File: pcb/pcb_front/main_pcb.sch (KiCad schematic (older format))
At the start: 31 parts, among them J1 AVR-ISP-6, J2 USB_C_Receptacle, Q1 Q_NMOS_DGS, SW1 RESET, SW2 BOOT, SW3 BL_STEP, U1 ATmega32-16PU, Y1 Crystal

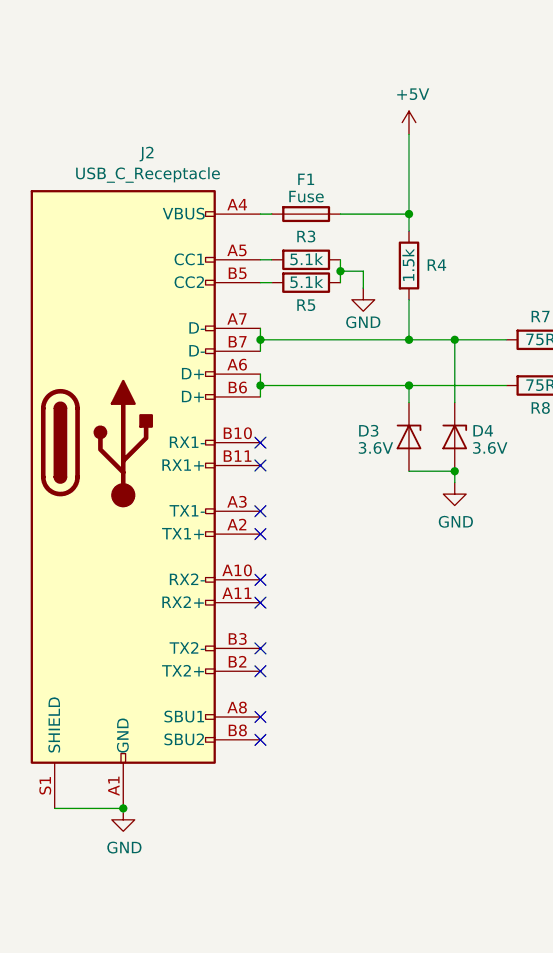
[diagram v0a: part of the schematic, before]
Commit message: Finish footprint assignments
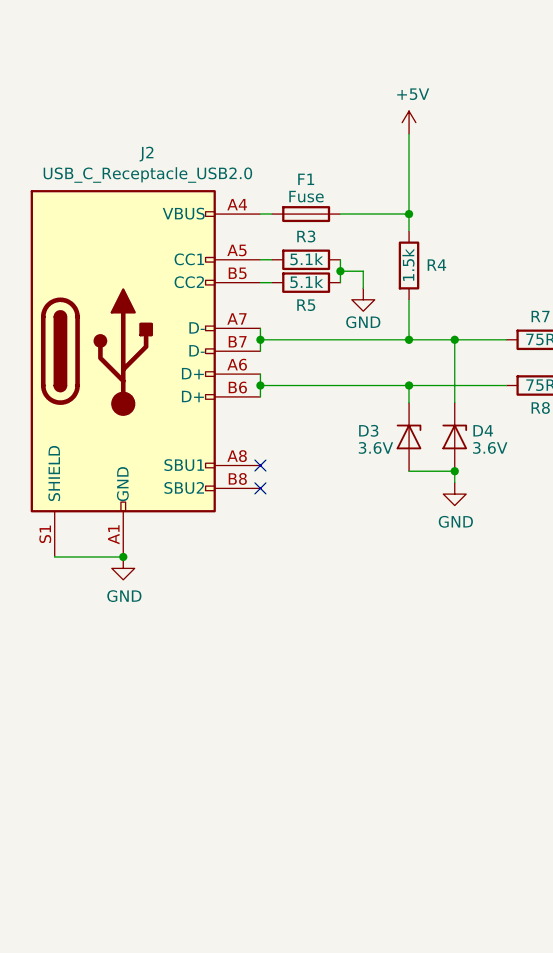
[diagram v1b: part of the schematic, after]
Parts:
- removed J2: USB_C_Receptacle, symbol Connector:USB_C_Receptacle
- added J2: USB_C_Receptacle_USB2.0, Connector_USB:USB_C_Receptacle_GCT_USB4085, symbol Connector:USB_C_Receptacle_USB2.0
- C1: footprint (none) -> Capacitor_THT:CP_Radial_D4.0mm_P1.50mm
- C2, C3: footprint (none) -> Capacitor_THT:C_Disc_D4.3mm_W1.9mm_P5.00mm
- C4, C5: footprint (none) -> Capacitor_THT:C_Disc_D3.0mm_W1.6mm_P2.50mm
- D1, D2, D5: footprint (none) -> LED_THT:LED_D3.0mm_Clear
- D3, D4, D6: footprint (none) -> Diode_THT:D_DO-35_SOD27_P7.62mm_Horizontal
- F1: footprint (none) -> Capacitor_THT:C_Disc_D5.0mm_W2.5mm_P5.00mm
- J1: footprint (none) -> Connector_PinHeader_2.54mm:PinHeader_2x03_P2.54mm_Vertical
- Q1: footprint (none) -> Package_TO_SOT_THT:TO-262-3_Vertical
- R1, R10, R11, R2, R3, R4, R5, R6, R7, R8, R9: footprint (none) -> Resistor_THT:R_Axial_DIN0204_L3.6mm_D1.6mm_P7.62mm_Horizontal
- SW1, SW2: footprint (none) -> Button_Switch_THT:SW_PUSH_6mm
- SW3: footprint (none) -> Button_Switch_THT:SW_Tactile_SPST_Angled_PTS645Vx31-2LFS
- Y1: footprint (none) -> Crystal:Crystal_HC49-4H_Vertical
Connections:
- net GND: now also J2.A1 (GND), J2.A12 (GND), J2.B1 (GND), J2.B12 (GND), J2.S1 (SHIELD)
- net at F1.2: now also J2.A4 (VBUS), J2.A9 (VBUS), J2.B4 (VBUS), J2.B9 (VBUS)
- net at R3.2: now also J2.A5 (CC1)
- net at D3.1 (K), R8.2: now also J2.A6 (D+), J2.B6 (D+)
- net at D4.1 (K), R4.2, R7.2: now also J2.A7 (D-), J2.B7 (D-)
- net at R5.2: now also J2.B5 (CC2)
- no-connect marks 11 -> 3
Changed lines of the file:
@@
 F 0 "Y1" H 4375 2525 50  0000 C CNN
 F 1 "Crystal" H 4375 2600 50  0000 C CNN
-F 2 "" H 4375 2750 50  0001 C CNN
+F 2 "Crystal:Crystal_HC49-4H_Vertical" H 4375 2750 50  0001 C CNN
 F 3 "~" H 4375 2750 50  0001 C CNN
 	1    4375 2750
@@
 F 0 "C4" H 3975 3000 50  0000 L CNN
 F 1 "22p" H 3925 2900 50  0000 L CNN
-F 2 "" H 4213 2800 50  0001 C CNN
+F 2 "Capacitor_THT:C_Disc_D3.0mm_W1.6mm_P2.50mm" H 4213 2800 50  0001 C CNN
 F 3 "~" H 4175 2950 50  0001 C CNN
 	1    4175 2950
@@
 F 0 "C5" H 4690 2996 50  0000 L CNN
 F 1 "22p" H 4690 2905 50  0000 L CNN
-F 2 "" H 4613 2800 50  0001 C CNN
+F 2 "Capacitor_THT:C_Disc_D3.0mm_W1.6mm_P2.50mm" H 4613 2800 50  0001 C CNN
 F 3 "~" H 4575 2950 50  0001 C CNN
 	1    4575 2950
@@
 F 0 "SW1" H 7975 5380 50  0000 C CNN
 F 1 "RESET" H 7975 5289 50  0000 C CNN
-F 2 "" H 7975 5125 60  0000 C CNN
+F 2 "Button_Switch_THT:SW_PUSH_6mm" H 7975 5125 60  0001 C CNN
 F 3 "" H 7975 5125 60  0000 C CNN
 	1    7975 5125
@@
 F 0 "SW2" H 7975 5905 50  0000 C CNN
 F 1 "BOOT" H 7975 5814 50  0000 C CNN
-F 2 "" H 7975 5650 60  0000 C CNN
+F 2 "Button_Switch_THT:SW_PUSH_6mm" H 7975 5650 60  0001 C CNN
 F 3 "" H 7975 5650 60  0000 C CNN
 	1    7975 5650
@@
 F 0 "R11" H 7475 4975 50  0000 L CNN
 F 1 "10k" V 7675 4900 50  0000 L CNN
-F 2 "" V 7605 4975 50  0001 C CNN
+F 2 "Resistor_THT:R_Axial_DIN0204_L3.6mm_D1.6mm_P7.62mm_Horizontal" V 7605 4975 50  0001 C CNN
 F 3 "~" H 7675 4975 50  0001 C CNN
 	1    7675 4975
@@
 F 0 "D5" H 7968 4095 50  0000 C CNN
 F 1 "POWER" H 7968 4186 50  0000 C CNN
-F 2 "" H 7975 4350 50  0001 C CNN
+F 2 "LED_THT:LED_D3.0mm_Clear" H 7975 4350 50  0001 C CNN
 F 3 "~" H 7975 4350 50  0001 C CNN
 	1    7975 4350
@@
 F 0 "D1" H 7968 3145 50  0000 C CNN
 F 1 "CAPSLOCK" H 7968 3236 50  0000 C CNN
-F 2 "" H 7975 3400 50  0001 C CNN
+F 2 "LED_THT:LED_D3.0mm_Clear" H 7975 3400 50  0001 C CNN
 F 3 "~" H 7975 3400 50  0001 C CNN
 	1    7975 3400
@@
 F 0 "R10" V 8175 4350 50  0000 C CNN
 F 1 "1.5k" V 8275 4350 50  0000 C CNN
-F 2 "" V 8205 4350 50  0001 C CNN
+F 2 "Resistor_THT:R_Axial_DIN0204_L3.6mm_D1.6mm_P7.62mm_Horizontal" V 8205 4350 50  0001 C CNN
 F 3 "~" H 8275 4350 50  0001 C CNN
 	1    8275 4350
@@
 F 0 "R6" V 8175 3400 50  0000 C CNN
 F 1 "1.5k" V 8275 3400 50  0000 C CNN
-F 2 "" V 8205 3400 50  0001 C CNN
+F 2 "Resistor_THT:R_Axial_DIN0204_L3.6mm_D1.6mm_P7.62mm_Horizontal" V 8205 3400 50  0001 C CNN
 F 3 "~" H 8275 3400 50  0001 C CNN
 	1    8275 3400
@@
 F 0 "J1" H 9571 3571 50  0000 R CNN
 F 1 "AVR-ISP-6" H 9571 3480 50  0000 R CNN
-F 2 "" V 9650 3525 50  0001 C CNN
+F 2 "Connector_PinHeader_2.54mm:PinHeader_2x03_P2.54mm_Vertical" V 9650 3525 50  0001 C CNN
 F 3 " ~" H 8625 2925 50  0001 C CNN
 	1    9900 3475
@@
 Text GLabel 7825 3400 0    50   Input ~ 0
 CAPSLOCK
-$Comp
-L Connector:USB_C_Receptacle J2
-U 1 1 612B5A26
-P 1775 4100
-F 0 "J2" H 1882 5367 50  0000 C CNN
-F 1 "USB_C_Receptacle" H 1882 5276 50  0000 C CNN
-F 2 "" H 1925 4100 50  0001 C CNN
-F 3 "https://www.usb.org/sites/default/files/documents/usb_type-c.zip" H 1925 4100 50  0001 C CNN
-	1    1775 4100
-	1    0    0    -1
-$EndComp
-NoConn ~ 2375 4400
-NoConn ~ 2375 4500
-NoConn ~ 2375 4700
-NoConn ~ 2375 4800
-NoConn ~ 2375 5000
-NoConn ~ 2375 5100
-NoConn ~ 2375 5300
-NoConn ~ 2375 5400
-Wire Wire Line
-	1475 5700 1775 5700
+Wire Wire Line
+	1475 4600 1775 4600
 $Comp
 L power:GND #PWR019
 U 1 1 612B93FC
-P 1775 5700
-F 0 "#PWR019" H 1775 5450 50  0001 C CNN
-F 1 "GND" H 1780 5527 50  0000 C CNN
-F 2 "" H 1775 5700 50  0001 C CNN
-F 3 "" H 1775 5700 50  0001 C CNN
-	1    1775 5700
-	1    0    0    -1
-$EndComp
-Connection ~ 1775 5700
-NoConn ~ 2375 4200
-NoConn ~ 2375 4100
+P 1775 4600
+F 0 "#PWR019" H 1775 4350 50  0001 C CNN
+F 1 "GND" H 1780 4427 50  0000 C CNN
+F 2 "" H 1775 4600 50  0001 C CNN
+F 3 "" H 1775 4600 50  0001 C CNN
+	1    1775 4600
+	1    0    0    -1
+$EndComp
 $Comp
 L Device:Fuse F1
@@
 F 0 "F1" V 2425 3100 50  0000 C CNN
 F 1 "Fuse" V 2500 3100 50  0000 C CNN
-F 2 "" V 2505 3100 50  0001 C CNN
+F 2 "Capacitor_THT:C_Disc_D5.0mm_W2.5mm_P5.00mm" V 2505 3100 50  0001 C CNN
 F 3 "~" H 2575 3100 50  0001 C CNN
 	1    2575 3100
@@
 F 0 "R3" V 2475 3300 50  0000 C CNN
 F 1 "5.1k" V 2575 3300 50  0000 C CNN
-F 2 "" V 2505 3300 50  0001 C CNN
+F 2 "Resistor_THT:R_Axial_DIN0204_L3.6mm_D1.6mm_P7.62mm_Horizontal" V 2505 3300 50  0001 C CNN
 F 3 "~" H 2575 3300 50  0001 C CNN
 	1    2575 3300
@@
 F 0 "R5" V 2675 3400 50  0000 C CNN
 F 1 "5.1k" V 2575 3400 50  0000 C CNN
-F 2 "" V 2505 3400 50  0001 C CNN
+F 2 "Resistor_THT:R_Axial_DIN0204_L3.6mm_D1.6mm_P7.62mm_Horizontal" V 2505 3400 50  0001 C CNN
 F 3 "~" H 2575 3400 50  0001 C CNN
 	1    2575 3400
@@
 F 0 "R7" V 3500 3650 50  0000 C CNN
 F 1 "75R" V 3600 3650 50  0000 C CNN
-F 2 "" V 3530 3650 50  0001 C CNN
+F 2 "Resistor_THT:R_Axial_DIN0204_L3.6mm_D1.6mm_P7.62mm_Horizontal" V 3530 3650 50  0001 C CNN
 F 3 "~" H 3600 3650 50  0001 C CNN
 	1    3600 3650
@@
 F 0 "R8" V 3700 3850 50  0000 C CNN
 F 1 "75R" V 3600 3850 50  0000 C CNN
-F 2 "" V 3530 3850 50  0001 C CNN
+F 2 "Resistor_THT:R_Axial_DIN0204_L3.6mm_D1.6mm_P7.62mm_Horizontal" V 3530 3850 50  0001 C CNN
 F 3 "~" H 3600 3850 50  0001 C CNN
 	1    3600 3850
@@
 F 0 "D4" V 3200 4150 50  0000 L CNN
 F 1 "3.6V" V 3275 4150 50  0000 L CNN
-F 2 "" H 3225 4075 50  0001 C CNN
+F 2 "Diode_THT:D_DO-35_SOD27_P7.62mm_Horizontal" H 3225 4075 50  0001 C CNN
 F 3 "~" H 3225 4075 50  0001 C CNN
 	1    3225 4075
@@
 F 0 "D3" V 3000 3850 50  0000 L CNN
 F 1 "3.6V" V 3075 3850 50  0000 L CNN
-F 2 "" H 3025 4075 50  0001 C CNN
+F 2 "Diode_THT:D_DO-35_SOD27_P7.62mm_Horizontal" H 3025 4075 50  0001 C CNN
 F 3 "~" H 3025 4075 50  0001 C CNN
 	1    3025 4075
@@
 F 0 "R4" H 3100 3325 50  0000 L CNN
 F 1 "1.5k" V 3025 3250 50  0000 L CNN
-F 2 "" V 2955 3325 50  0001 C CNN
+F 2 "Resistor_THT:R_Axial_DIN0204_L3.6mm_D1.6mm_P7.62mm_Horizontal" V 2955 3325 50  0001 C CNN
 F 3 "~" H 3025 3325 50  0001 C CNN
 	1    3025 3325
@@
 F 0 "Q1" H 8204 2446 50  0000 L CNN
 F 1 "Q_NMOS_DGS" H 8204 2355 50  0000 L CNN
-F 2 "" H 8200 2500 50  0001 C CNN
+F 2 "Package_TO_SOT_THT:TO-262-3_Vertical" H 8200 2500 50  0001 C CNN
 F 3 "~" H 8000 2400 50  0001 C CNN
 	1    8000 2400
@@
 F 0 "R2" H 7825 2600 50  0000 L CNN
 F 1 "10k" V 7750 2525 50  0000 L CNN
-F 2 "" V 7680 2600 50  0001 C CNN
+F 2 "Resistor_THT:R_Axial_DIN0204_L3.6mm_D1.6mm_P7.62mm_Horizontal" V 7680 2600 50  0001 C CNN
 F 3 "~" H 7750 2600 50  0001 C CNN
 	1    7750 2600
@@
 F 0 "R1" V 7450 2400 50  0000 C CNN
 F 1 "470" V 7550 2400 50  0000 C CNN
-F 2 "" V 7480 2400 50  0001 C CNN
+F 2 "Resistor_THT:R_Axial_DIN0204_L3.6mm_D1.6mm_P7.62mm_Horizontal" V 7480 2400 50  0001 C CNN
 F 3 "~" H 7550 2400 50  0001 C CNN
 	1    7550 2400
@@
 F 0 "SW3" H 7975 6455 50  0000 C CNN
 F 1 "BL_STEP" H 7975 6364 50  0000 C CNN
-F 2 "" H 7975 6200 60  0000 C CNN
+F 2 "Button_Switch_THT:SW_Tactile_SPST_Angled_PTS645Vx31-2LFS" H 7975 6200 60  0001 C CNN
 F 3 "" H 7975 6200 60  0000 C CNN
 	1    7975 6200
@@
 F 0 "D6" H 8425 5984 50  0000 C CNN
 F 1 "1N4148" H 8425 6075 50  0000 C CNN
-F 2 "" H 8425 6200 50  0001 C CNN
+F 2 "Diode_THT:D_DO-35_SOD27_P7.62mm_Horizontal" H 8425 6200 50  0001 C CNN
 F 3 "~" H 8425 6200 50  0001 C CNN
 	1    8425 6200
@@
 F 0 "C3" H 8225 1350 50  0000 L CNN
 F 1 "0.1u" H 8200 950 50  0000 L CNN
-F 2 "" H 8313 1000 50  0001 C CNN
+F 2 "Capacitor_THT:C_Disc_D4.3mm_W1.9mm_P5.00mm" H 8313 1000 50  0001 C CNN
 F 3 "~" H 8275 1150 50  0001 C CNN
 	1    8275 1150
@@
 F 0 "C2" H 8025 1350 50  0000 L CNN
 F 1 "0.1u" H 8000 950 50  0000 L CNN
-F 2 "" H 8113 1000 50  0001 C CNN
+F 2 "Capacitor_THT:C_Disc_D4.3mm_W1.9mm_P5.00mm" H 8113 1000 50  0001 C CNN
 F 3 "~" H 8075 1150 50  0001 C CNN
 	1    8075 1150
@@
 F 0 "C1" H 7825 1350 50  0000 L CNN
 F 1 "4.7u" H 7800 950 50  0000 L CNN
-F 2 "" H 7875 1150 50  0001 C CNN
+F 2 "Capacitor_THT:CP_Radial_D4.0mm_P1.50mm" H 7875 1150 50  0001 C CNN
 F 3 "~" H 7875 1150 50  0001 C CNN
 	1    7875 1150
@@
 F 0 "D2" H 7968 3620 50  0000 C CNN
 F 1 "NUMLOCK" H 7968 3711 50  0000 C CNN
-F 2 "" H 7975 3875 50  0001 C CNN
+F 2 "LED_THT:LED_D3.0mm_Clear" H 7975 3875 50  0001 C CNN
 F 3 "~" H 7975 3875 50  0001 C CNN
 	1    7975 3875
@@
 F 0 "R9" V 8175 3875 50  0000 C CNN
 F 1 "1.5k" V 8275 3875 50  0000 C CNN
-F 2 "" V 8205 3875 50  0001 C CNN
+F 2 "Resistor_THT:R_Axial_DIN0204_L3.6mm_D1.6mm_P7.62mm_Horizontal" V 8205 3875 50  0001 C CNN
 F 3 "~" H 8275 3875 50  0001 C CNN
 	1    8275 3875
@@
 Text GLabel 7825 3875 0    50   Input ~ 0
 NUMLOCK
+$Comp
+L Connector:USB_C_Receptacle_USB2.0 J2
+U 1 1 6129B621
+P 1775 3700
+F 0 "J2" H 1882 4567 50  0000 C CNN
+F 1 "USB_C_Receptacle_USB2.0" H 1882 4476 50  0000 C CNN
+F 2 "Connector_USB:USB_C_Receptacle_GCT_USB4085" H 1925 3700 50  0001 C CNN
+F 3 "https://www.usb.org/sites/default/files/documents/usb_type-c.zip" H 1925 3700 50  0001 C CNN
+	1    1775 3700
+	1    0    0    -1
+$EndComp
+Connection ~ 1775 4600
+NoConn ~ 2375 4200
+NoConn ~ 2375 4300
 $EndSCHEMATC
